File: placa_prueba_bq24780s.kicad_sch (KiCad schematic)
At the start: 1 part, among them U1 BQ24780SRUYR

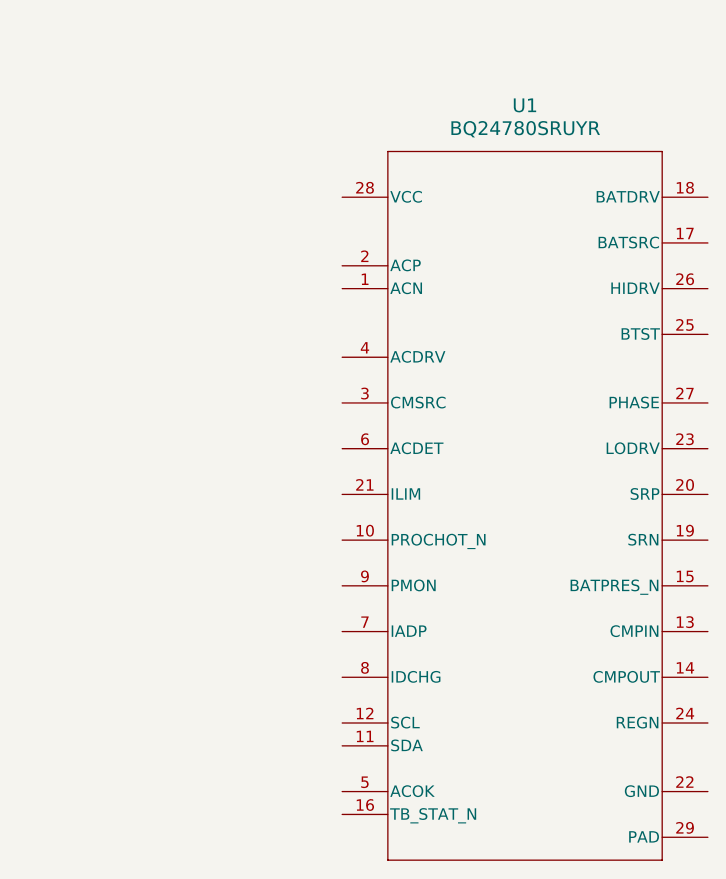
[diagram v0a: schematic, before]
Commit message: Avances en el esquemático.
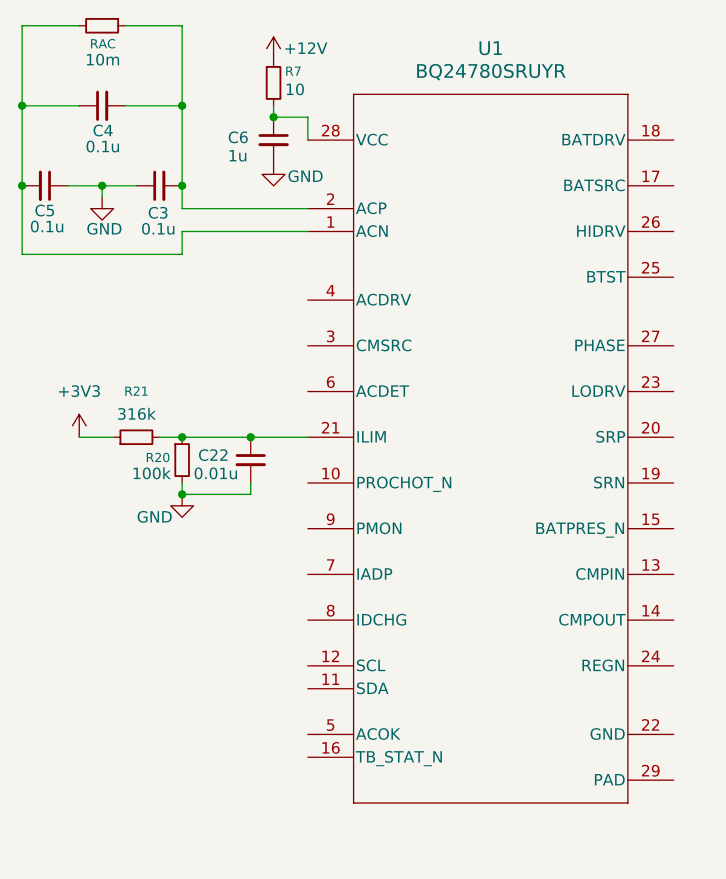
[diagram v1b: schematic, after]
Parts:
- added C22: 0.01u, symbol Device:C_Small
- added C3, C4, C5: 0.1u, symbol Device:C_Small
- added C6: 1u, symbol Device:C_Small
- added R20: 100k, symbol Device:R_Small
- added R21: 316k, symbol Device:R_Small
- added R7: 10, symbol Device:R_Small
- added RAC: 10m, symbol Device:R_Small
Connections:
- net at U1.1 (ACN): now also C4.1, C5.2, RAC.2
- net at U1.2 (ACP): now also C3.2, C4.2, RAC.1
- net at U1.21 (ILIM): now also C22.1, R20.1, R21.2
- net at U1.28 (VCC): now also C6.1, R7.2
- new net +12V: R7.1
- new net +3V3: R21.1
- new net GND: C22.2, C3.1, C5.1, C6.2, R20.2
